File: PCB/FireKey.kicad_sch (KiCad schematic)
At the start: 76 parts, among them SW1 SW_MEC_5E, U1 Arduino_Pro_Micro_USB-C

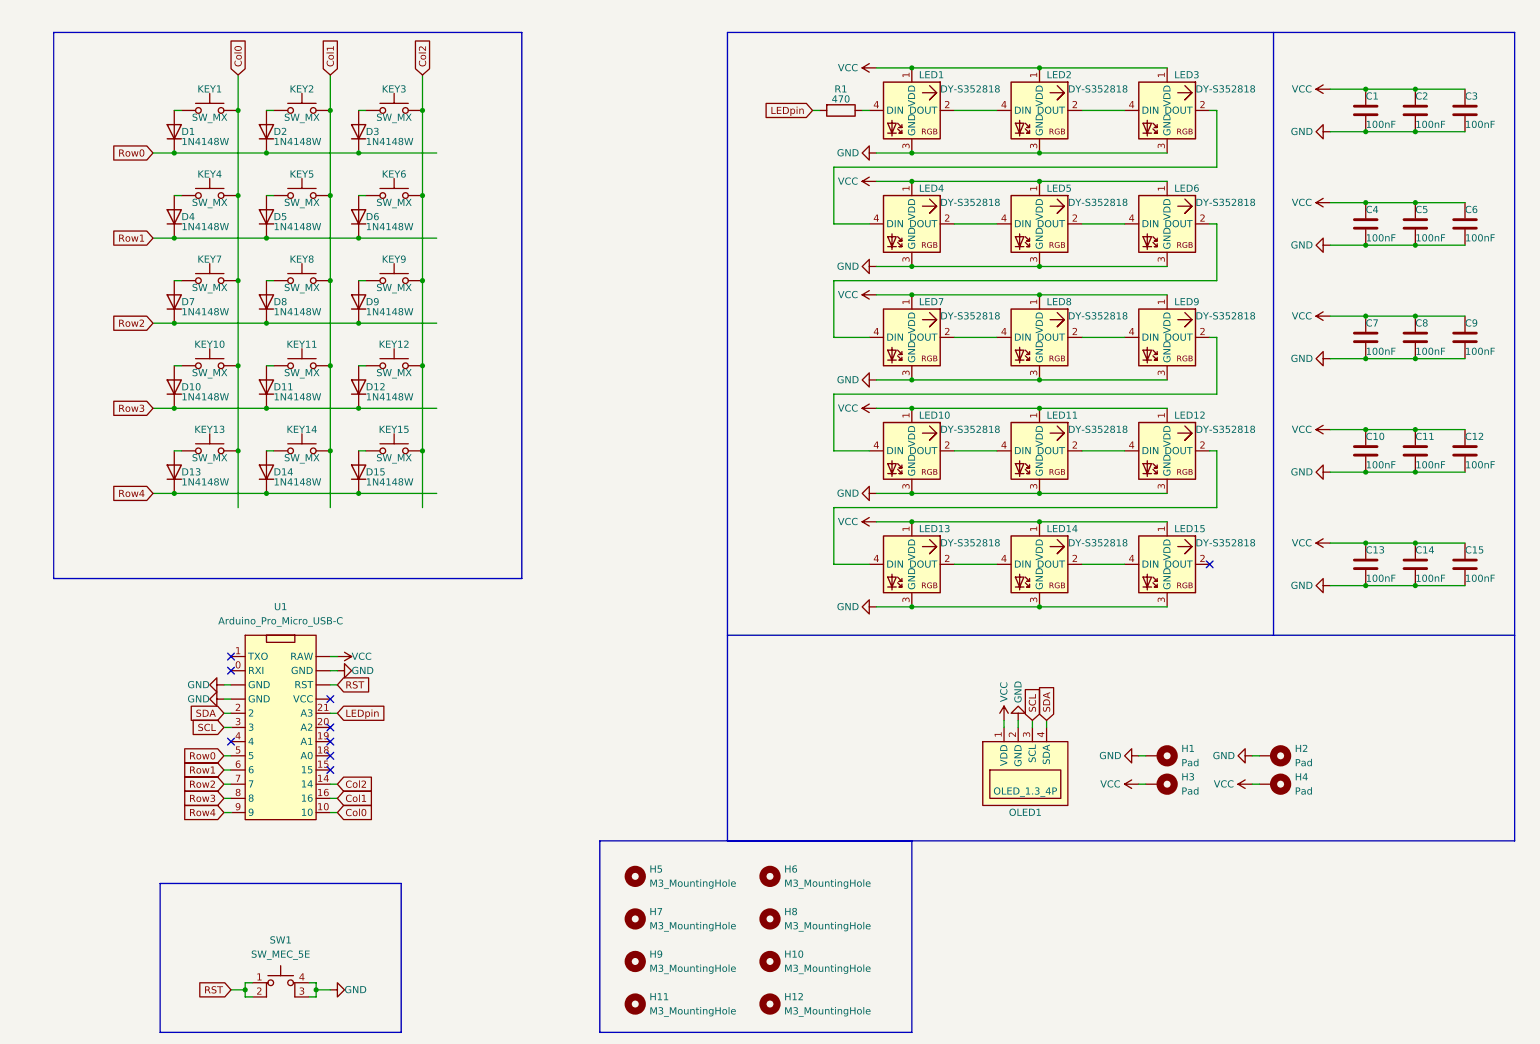
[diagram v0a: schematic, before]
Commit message: worked on schematic structure
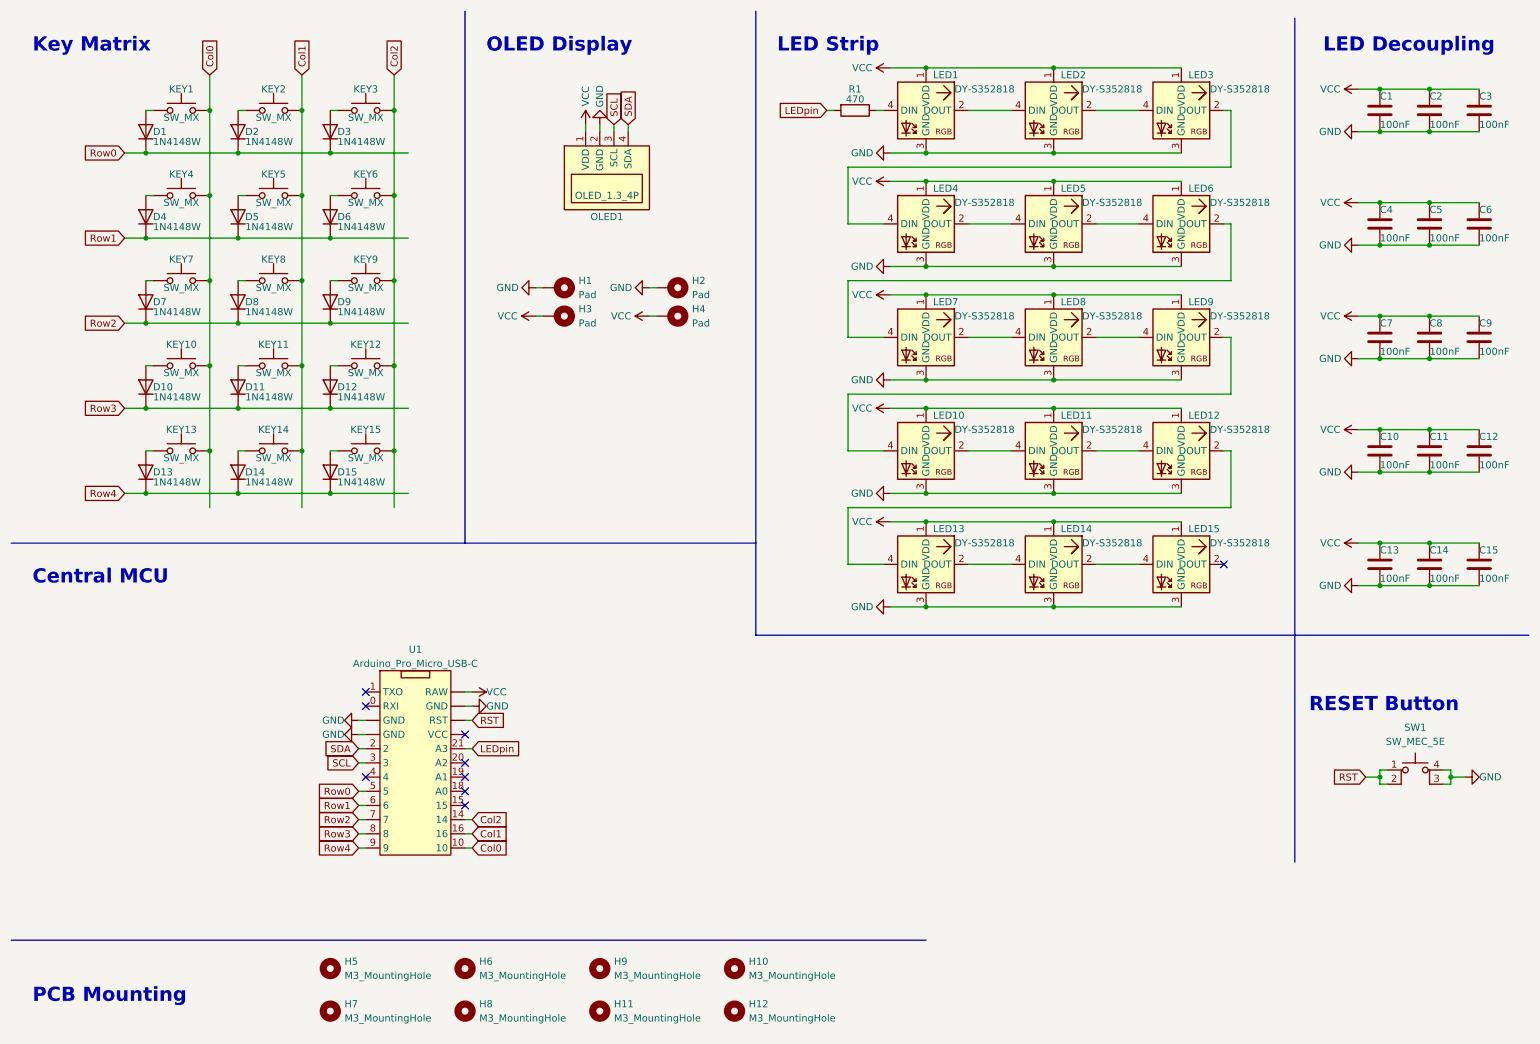
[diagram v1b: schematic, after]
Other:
- note added: "Central MCU"
- note added: "Key Matrix"
- note added: "LED Decoupling"
- note added: "LED Strip"
- note added: "OLED Display"
- note added: "PCB Mounting"
- note added: "RESET Button"
- moved on the sheet: C1, C10, C11, C12, C13, C14, C15, C2, C3, C4, C5, C6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
